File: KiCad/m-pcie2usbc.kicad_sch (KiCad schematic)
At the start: 6 parts

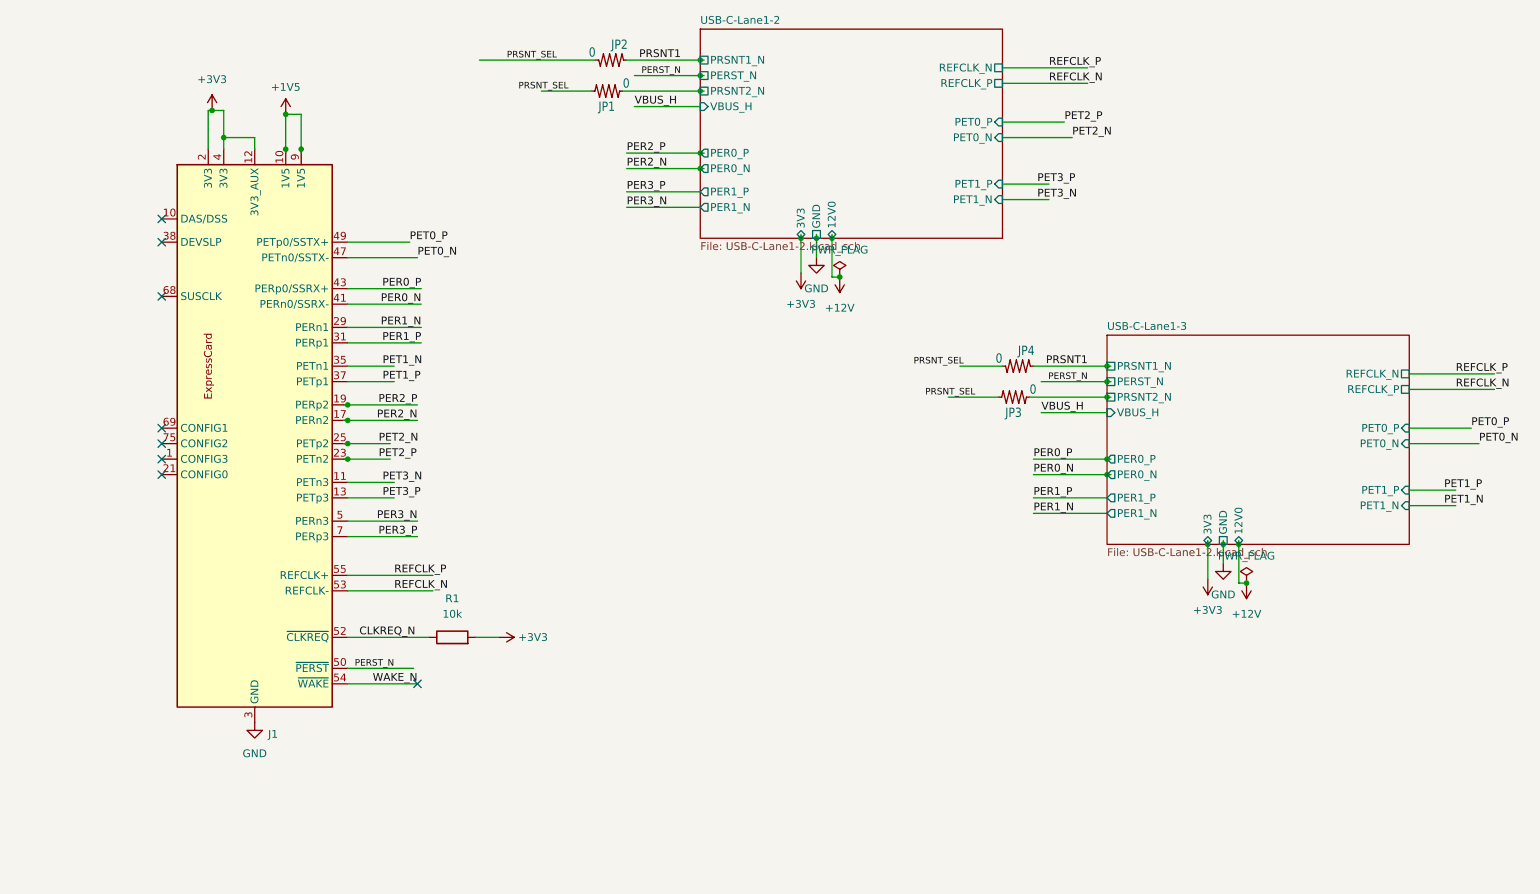
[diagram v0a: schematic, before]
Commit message: WIP - fine tune routing
WIP - fine tune routing
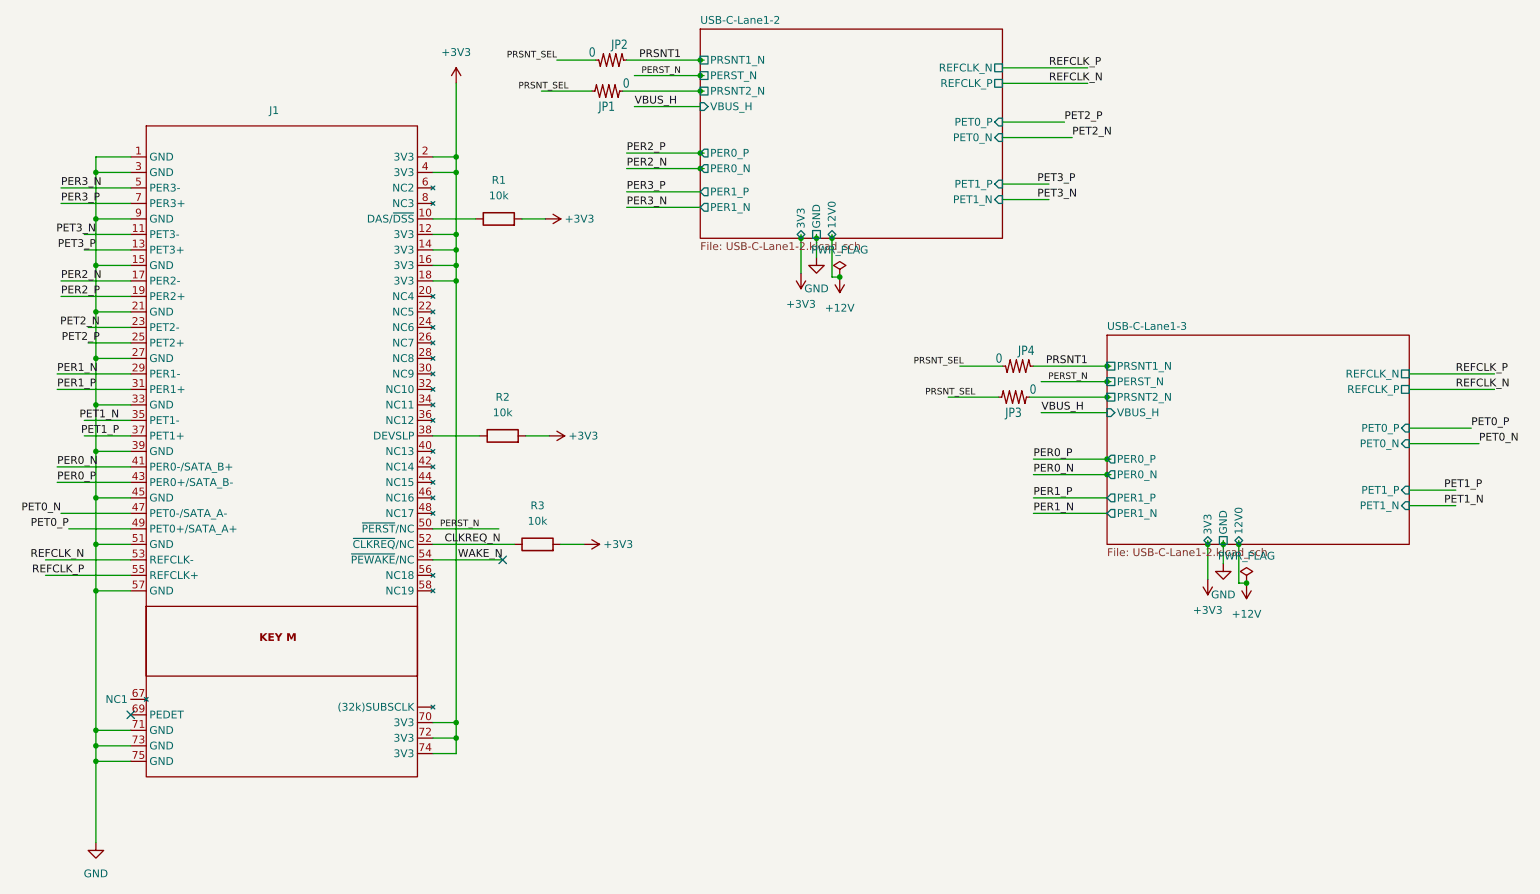
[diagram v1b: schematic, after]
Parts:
- removed J1: ~, mpcie:mpcie-full-card, symbol Connector:M.2-key-M
- added J1: ~, M.2-Templates:M.2-M-KEY, symbol M.2-Templates-eagle-import:M.2-M-Key
- added R1, R2: 10k, Resistor_SMD:R_0201_0603Metric_Pad0.64x0.40mm_HandSolder, symbol Device:R
- renumbered R1 to R3
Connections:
- net +3V3: now also J1.12 (3V3), J1.14 (3V3), J1.16 (3V3), J1.18 (3V3), J1.2 (3V3), J1.4 (3V3), J1.70 (3V3), J1.72 (3V3), J1.74 (3V3), R1.2, R2.2
- net CLKREQ_N: now also J1.52 (~{CLKREQ}/NC)
- net GND: now also J1.1 (GND), J1.11 (PET3-), J1.13 (PET3+), J1.15 (GND), J1.21 (GND), J1.27 (GND), J1.3 (GND), J1.33 (GND), J1.39 (GND), J1.45 (GND), J1.51 (GND), J1.57 (GND), J1.71 (GND), J1.73 (GND), J1.75 (GND), J1.9 (GND)
- net PER0_N: now also J1.41 (PER0-/SATA_B+)
- net PER0_P: now also J1.43 (PER0+/SATA_B-)
- net PER1_N: now also J1.29 (PER1-)
- net PER1_P: now also J1.31 (PER1+)
- net PER2_N: now also J1.17 (PER2-)
- net PER2_P: now also J1.19 (PER2+)
- net PER3_N: now also J1.5 (PER3-)
- net PER3_P: now also J1.7 (PER3+)
- net PERST_N: now also J1.50 (~{PERST}/NC)
- net PET0_N: now also J1.47 (PET0-/SATA_A-)
- net PET0_P: now also J1.49 (PET0+/SATA_A+)
- net PET1_N: now also J1.35 (PET1-)
- net PET1_P: now also J1.37 (PET1+)
- net PET2_N: now also J1.23 (PET2-)
- net PET2_P: now also J1.25 (PET2+)
- net REFCLK_N: now also J1.53 (REFCLK-)
- net REFCLK_P: now also J1.55 (REFCLK+)
- net WAKE_N: now also J1.54 (~{PEWAKE}/NC)
- new net: J1.10 (DAS/~{DSS}), R1.1
- new net: J1.38 (DEVSLP), R2.1
- no-connect marks 8 -> 2
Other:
- moved on the sheet: R3

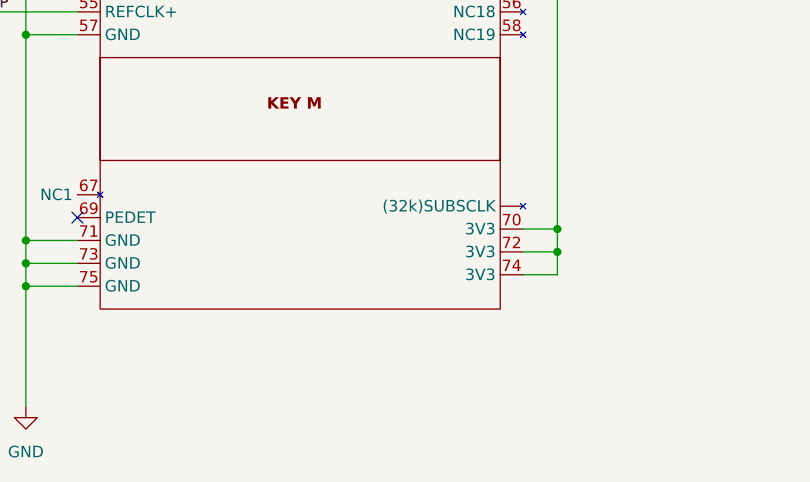
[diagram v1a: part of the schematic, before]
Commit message: Layout completed
Layout completed
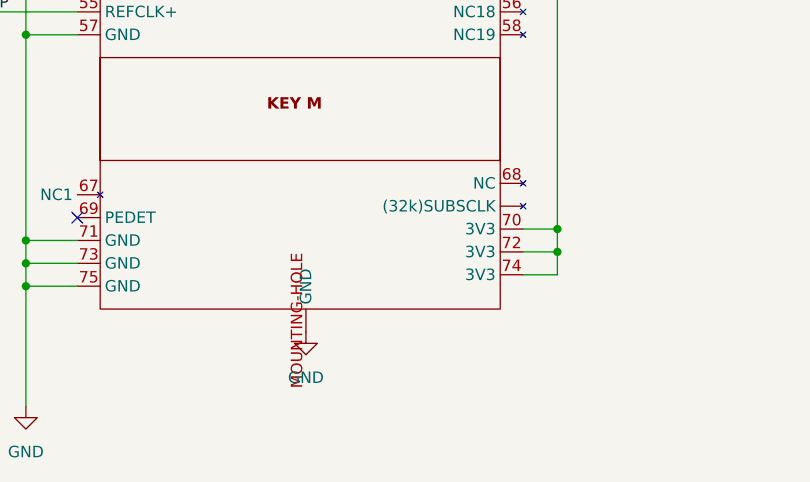
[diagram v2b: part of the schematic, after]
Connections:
- net GND: now also J1.MOUNTING-HOLE (GND)
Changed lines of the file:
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@@
     (pin "6")
     (pin "67")
+    (pin "68")
     (pin "69")
     (pin "7")
@@
     (pin "9")
     (pin "1")
+    (pin "MOUNTING-HOLE")
     (instances
       (project "m-pcie2usbc"
@@
         )
       )
+    )
+  )
+  (symbol (lib_id "power:GND") (at 66.04 172.72 0) (unit 1)
+    (in_bom yes) (on_board yes) (dnp no) (fields_autoplaced)
+    (property "Reference" "#PWR015" (at 66.04 179.07 0)
+      (effects (font (size 1.27 1.27)) hide)
+    )
+    (property "Value" "GND" (at 66.04 177.8 0)
+      (effects (font (size 1.27 1.27)))
+    )
+    (property "Footprint" "" (at 66.04 172.72 0)
+      (effects (font (size 1.27 1.27)) hide)
+    )
+    (property "Datasheet" "" (at 66.04 172.72 0)
+      (effects (font (size 1.27 1.27)) hide)
+    )
+    (pin "1")
+    (instances
+      (project "m-pcie2usbc"
+        (path "/c6966a4c-26ab-49f3-b12b-daf57b153bc7"
+          (reference "#PWR015") (unit 1)
+        )
+      )
